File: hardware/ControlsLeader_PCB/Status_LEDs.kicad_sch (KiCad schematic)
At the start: 25 parts, among them J5 BPS_Fault_LED

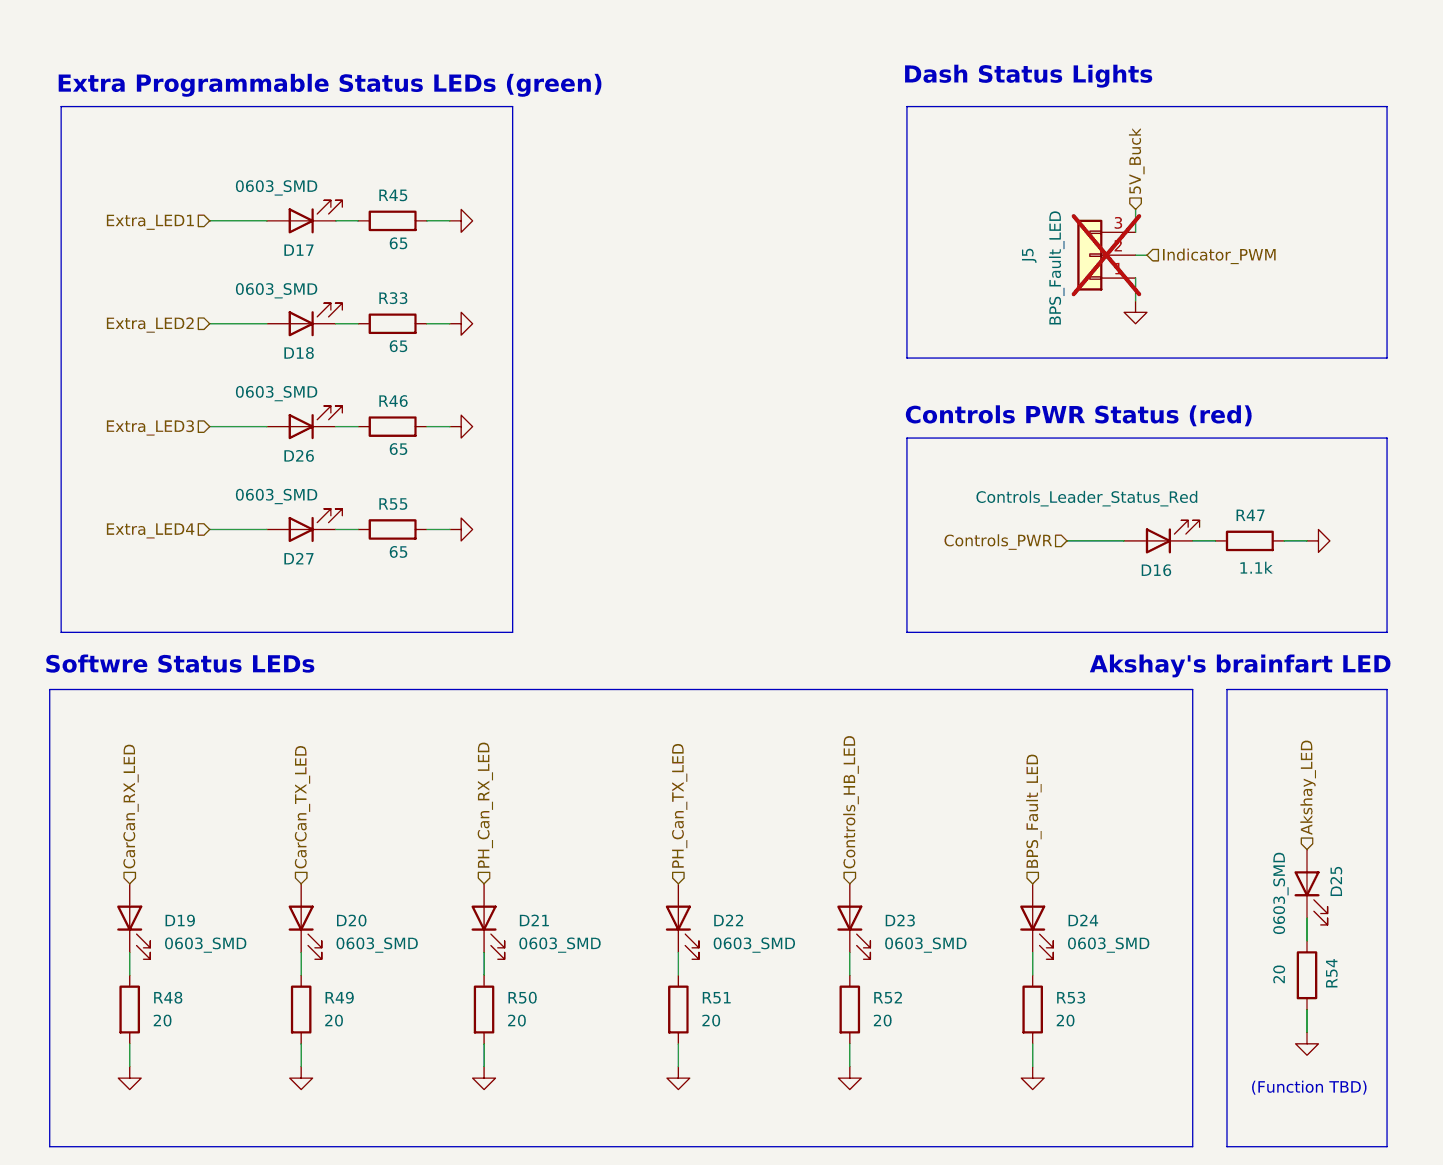
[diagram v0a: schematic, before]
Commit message: Mika is quite smart (#12)
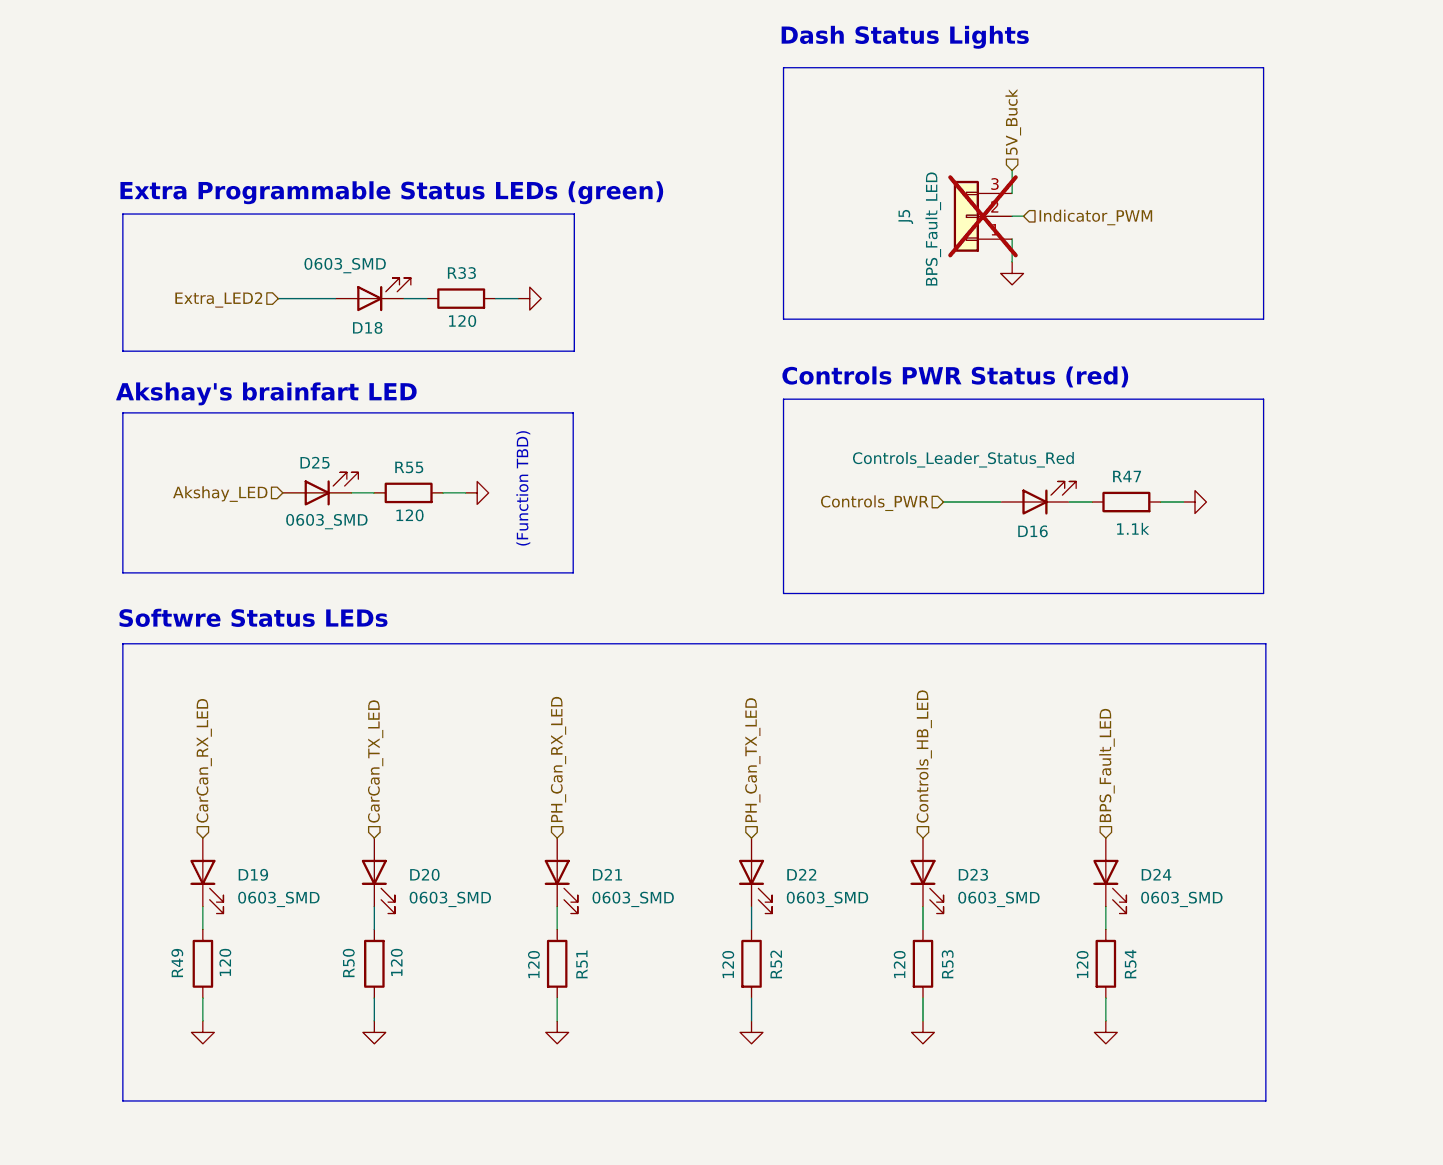
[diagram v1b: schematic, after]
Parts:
- removed D17, D26, D27: 0603_SMD, LED_SMD:LED_0603_1608Metric_Pad1.05x0.95mm_HandSolder, symbol Device:LED
- removed R45, R46: 65, Resistor_SMD:R_0603_1608Metric_Pad0.98x0.95mm_HandSolder, symbol Device:R
- removed R48: 20, Resistor_SMD:R_0603_1608Metric_Pad0.98x0.95mm_HandSolder, symbol Device:R
- R33, R55: value 65 -> 120
- R49, R50, R51, R52, R53, R54: value 20 -> 120; P/N ERJ-UP6D20R0V -> FC0402E65R0BGT0
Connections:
- net GND: now also R49.1, R50.1; no longer R49.2, R50.2
- net at R52.1: now also D22.1 (K); no longer D23.1 (K)
- net at D25.1 (K): now also R55.1; no longer R54.1
- net at D21.1 (K): now also R51.1; no longer R50.1
- net at D19.1 (K): now also R49.2
- net at D20.1 (K): now also R50.2; no longer R49.1
- net at D24.1 (K): now also R54.1; no longer R53.1
- new net: D23.1 (K), R53.1
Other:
- moved on the sheet: D16, D18, D19, D20, D21, D22, D23, D24, D25, J5, R47
